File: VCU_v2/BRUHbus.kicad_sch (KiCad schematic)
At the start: 22 parts, among them J3 BRUHBus, J4 BRUHBus, J5 BRUHBus, Q2 BSD235NH6327XT, Q3 BSD235NH6327XT

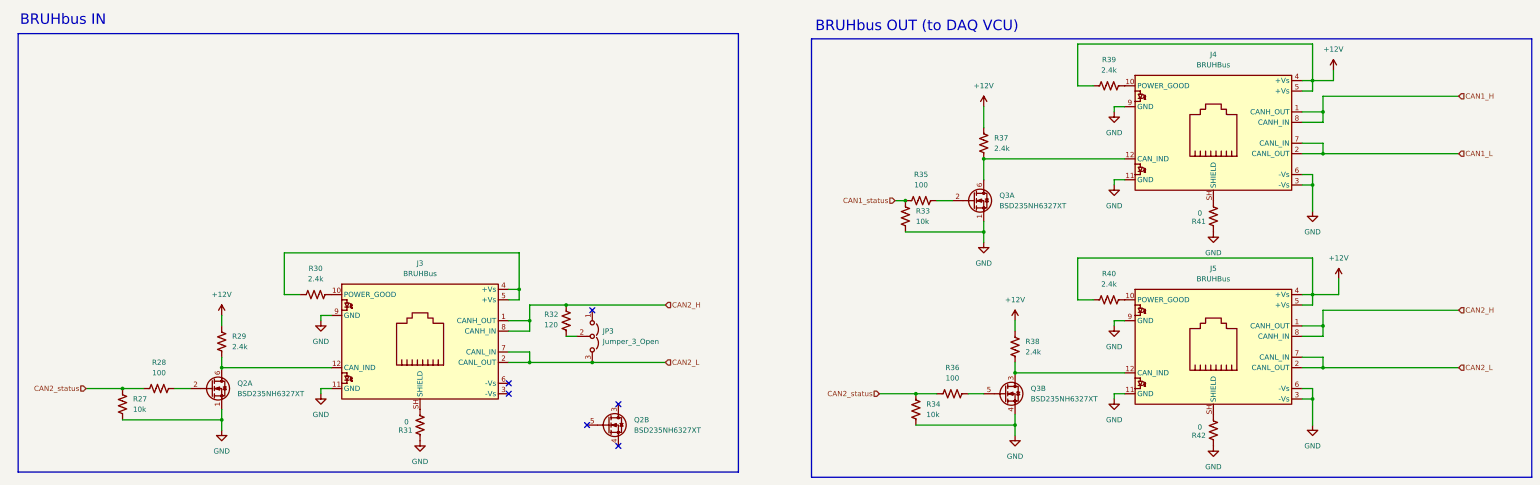
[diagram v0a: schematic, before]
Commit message: placements friggin 80% friggin done shoutout epstein
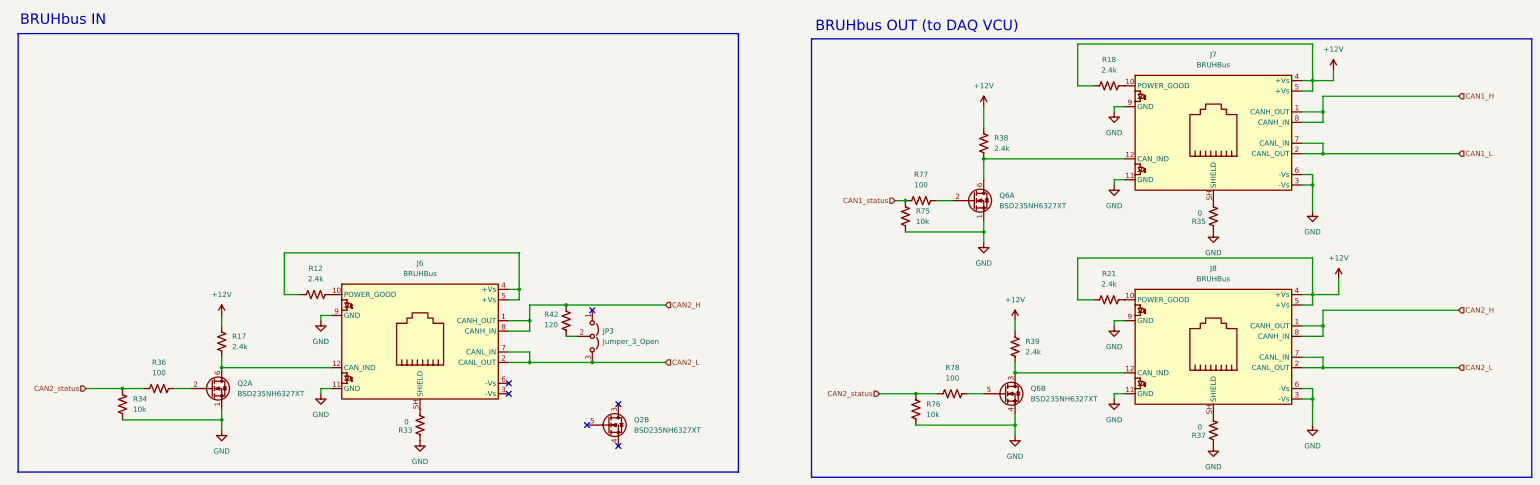
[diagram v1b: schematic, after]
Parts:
- renumbered J3 to J6, J4 to J7, J5 to J8, Q3 to Q6, R30 to R12, R29 to R17, R39 to R18, R40 to R21, R31 to R33, R27 to R34, R41 to R35, R28 to R36, R42 to R37, R37 to R38, R38 to R39, R32 to R42, R33 to R75, R34 to R76, R35 to R77, R36 to R78

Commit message: vcu v2 schematics done
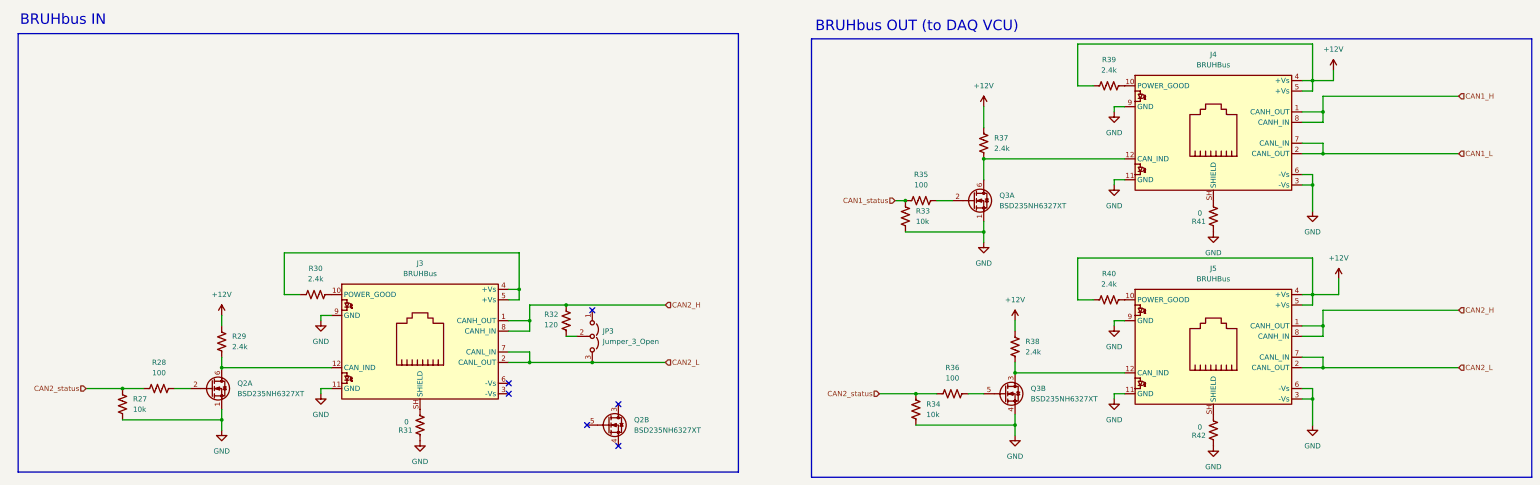
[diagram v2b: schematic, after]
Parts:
- renumbered J6 to J3, J7 to J4, J8 to J5, Q6 to Q3, R34 to R27, R36 to R28, R17 to R29, R12 to R30, R33 to R31, R42 to R32, R75 to R33, R76 to R34, R77 to R35, R78 to R36, R38 to R37, R39 to R38, R18 to R39, R21 to R40, R35 to R41, R37 to R42
